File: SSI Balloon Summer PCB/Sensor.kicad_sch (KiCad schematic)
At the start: 16 parts, among them J8 PT1000 Sensor, U10 MS5611-01BA03, U4 ICM-42688-P, U9 MAX31865ATP_T

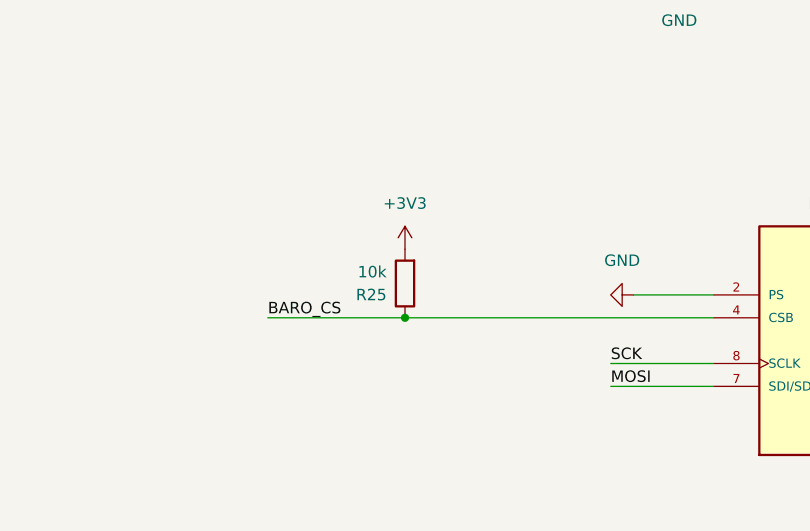
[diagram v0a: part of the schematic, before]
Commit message: Edits to PCB placement + traces - RF and GPS next
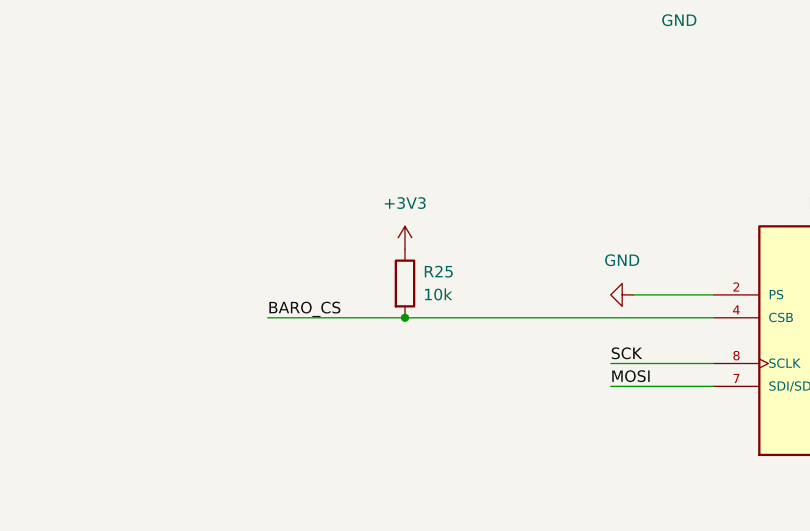
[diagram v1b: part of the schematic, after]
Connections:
- net +3V3: now also R25.1; no longer R25.2
- net BARO_CS: now also R25.2; no longer R25.1
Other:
- moved on the sheet: R25
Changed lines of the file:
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@@
+	)
+	(junction
+		(at 77.47 151.13)
+		(diameter 0)
+		(color 0 0 0 0)
 	)
 	(junction
@@
 	)
 	(junction
-		(at 77.47 151.13)
-		(diameter 0)
-		(color 0 0 0 0)
-	)
-	(junction
 		(at 123.19 86.36)
 		(diameter 0)
@@
 	(wire
 		(pts
+			(xy 77.47 151.13) (xy 111.76 151.13)
+		)
+		(stroke
+			(width 0)
+			(type default)
+		)
+	)
+	(wire
+		(pts
 			(xy 210.82 87.63) (xy 217.17 87.63)
 		)
@@
 		(pts
 			(xy 35.56 96.52) (xy 35.56 97.79)
-		)
-		(stroke
-			(width 0)
-			(type default)
-		)
-	)
-	(wire
-		(pts
-			(xy 77.47 151.13) (xy 111.76 151.13)
 		)
 		(stroke
@@
 	(symbol
 		(lib_id "Device:R")
-		(at 77.47 147.32 180)
+		(at 77.47 147.32 0)
 		(unit 1)
 		(body_style 1)
@@
 		(dnp no)
 		(property "Reference" "R25"
-			(at 75.438 148.59 0)
+			(at 79.502 146.05 0)
 			(show_name no)
 			(do_not_autoplace no)
@@
 		)
 		(property "Value" "10k"
-			(at 75.438 146.05 0)
+			(at 79.502 148.59 0)
 			(show_name no)
 			(do_not_autoplace no)
@@
 		)
 		(property "Footprint" "Resistor_SMD:R_0603_1608Metric"
-			(at 79.248 147.32 90)
-			(hide yes)
-			(show_name no)
+			(at 75.692 147.32 90)
+			(hide yes)
+			(show_name no)
